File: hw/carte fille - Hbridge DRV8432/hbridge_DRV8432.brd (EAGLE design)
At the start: 50 x 40 mm, 37 parts, among them IC1 DRV8402

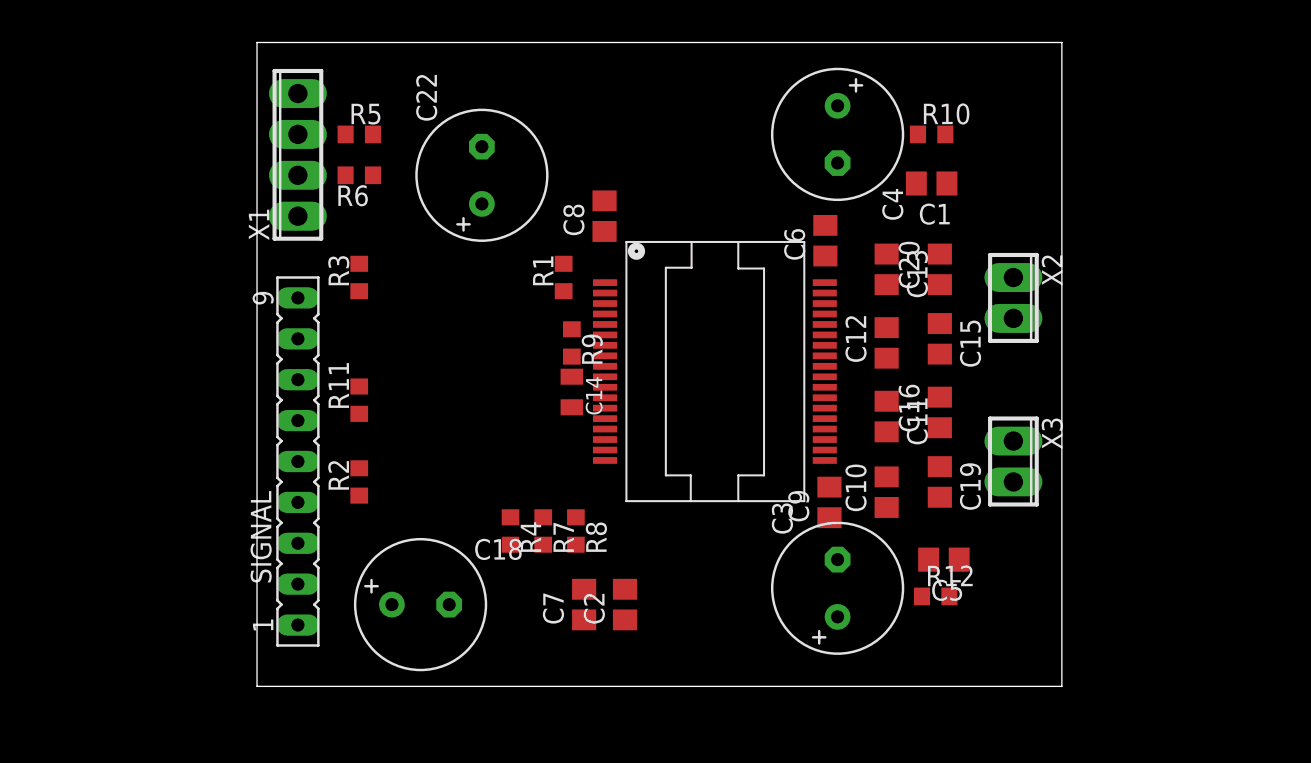
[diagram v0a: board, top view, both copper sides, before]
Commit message: Start routing the board
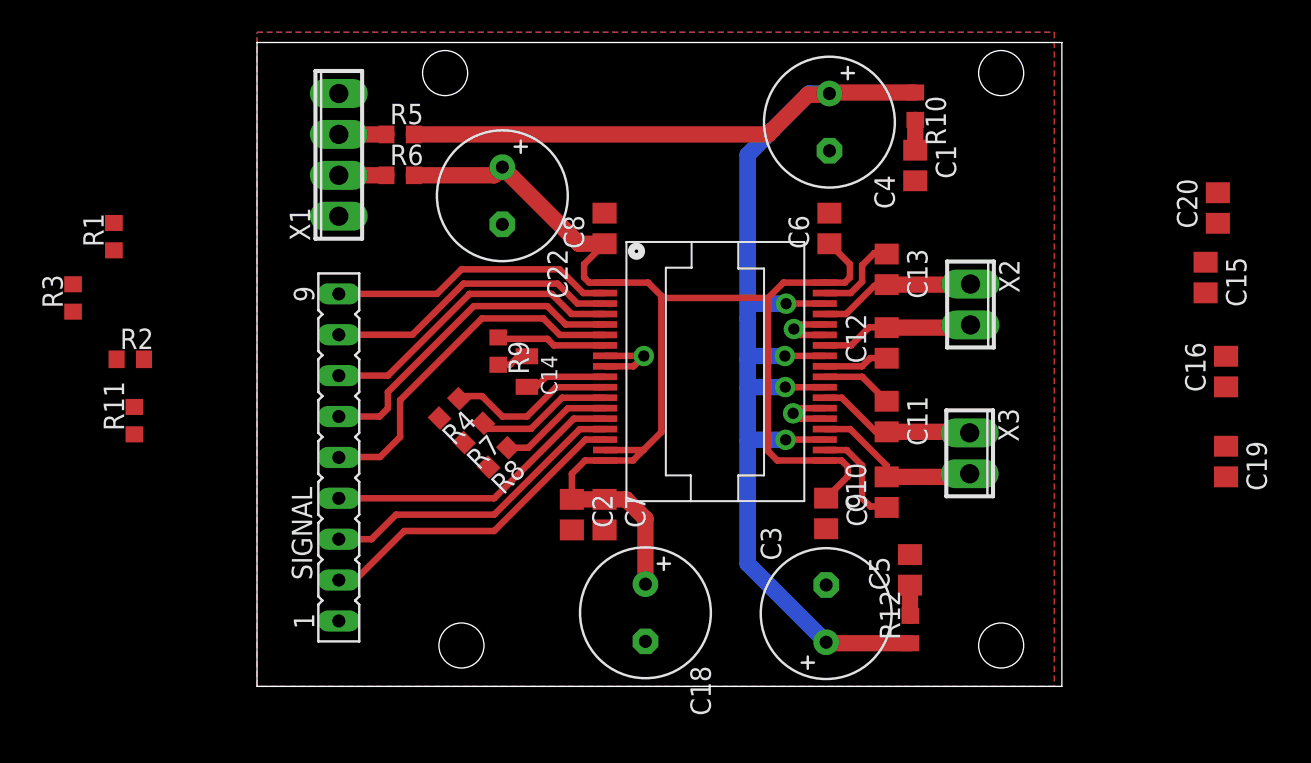
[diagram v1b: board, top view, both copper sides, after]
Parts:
- moved R1 28.1 mm to (-8.89, 27.9)
- moved C16 18.0 mm to (60.2, 19.6)
- moved C19 17.8 mm to (60.2, 14.0)
- moved R3 17.8 mm to (-11.4, 24.1)
- moved C20 17.7 mm to (59.7, 29.7)
- moved C15 16.9 mm to (58.9, 25.4)
- moved R2 16.1 mm to (-7.87, 20.3), turned to 0 degrees
- moved R11 14.0 mm to (-7.62, 16.5)
- moved C18 14.0 mm to (24.1, 4.57), turned to 270 degrees
- moved R4 8.52 mm to (11.9, 17.3), turned to 225 degrees
- moved R7 7.47 mm to (13.5, 15.7), turned to 225 degrees
- moved R8 6.65 mm to (15.0, 14.2), turned to 225 degrees
- moved C2 6.49 mm to (19.6, 10.7), turned to 270 degrees
- moved C7 5.73 mm to (21.6, 10.7), turned to 270 degrees
- moved R9 4.60 mm to (15.0, 20.8)
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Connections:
- net GND: no longer C15.1, C16.1, C19.1, C20.1
- net GVDD: no longer R1.2, R11.2, R2.2, R3.2
- net N$1: no longer R3.1
- net N$16: now also IC1.P$5; no longer IC1.P$15, R11.1
- net N$17: now also IC1.P$6; no longer IC1.P$4
- net N$18: now also IC1.P$14; no longer IC1.P$6
- net N$19: now also IC1.P$15; no longer IC1.P$14
- net N$6: no longer R2.1
- net N$8: now also IC1.P$4; no longer IC1.P$5, R1.1
- net PVDD: no longer C15.2, C16.2, C19.2, C20.2
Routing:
- net PVDD: track 0.00 -> 96.0 mm, vias 0 -> 4
- net GVDD: track 0.00 -> 83.7 mm
- net N$17: track 0.00 -> 21.9 mm
- net N$16: track 0.00 -> 20.5 mm
- net N$20: track 0.00 -> 20.2 mm
- net N$19: track 0.00 -> 19.4 mm
- net N$8: track 0.00 -> 19.2 mm
- net N$18: track 0.00 -> 18.6 mm
- net N$6: track 0.00 -> 18.4 mm
- net N$1: track 0.00 -> 17.8 mm
- net GND: track 0.00 -> 16.4 mm, vias 0 -> 3
- net OUT_D: track 0.00 -> 10.8 mm
- net N$5: track 0.00 -> 10.4 mm
- net OUT_C: track 0.00 -> 10.0 mm
- net OUT_A: track 0.00 -> 9.84 mm
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- added copper zone on layer 1, net GND
- added copper zone on layer 16, net GND
